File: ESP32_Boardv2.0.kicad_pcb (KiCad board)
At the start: 2 copper layers, 36 parts, among them IC1 AMS1117-3.3, IC2 CP2102N-A01-GQFN28, J1 USB_B_Micro, J2 Conn_01x19_Male, J3 Conn_01x19_Male, Q1 SS8050-G, Q2 SS8050-G, SW1 SW_Push, SW2 SW_Push, U1 ESP32-WROOM-32

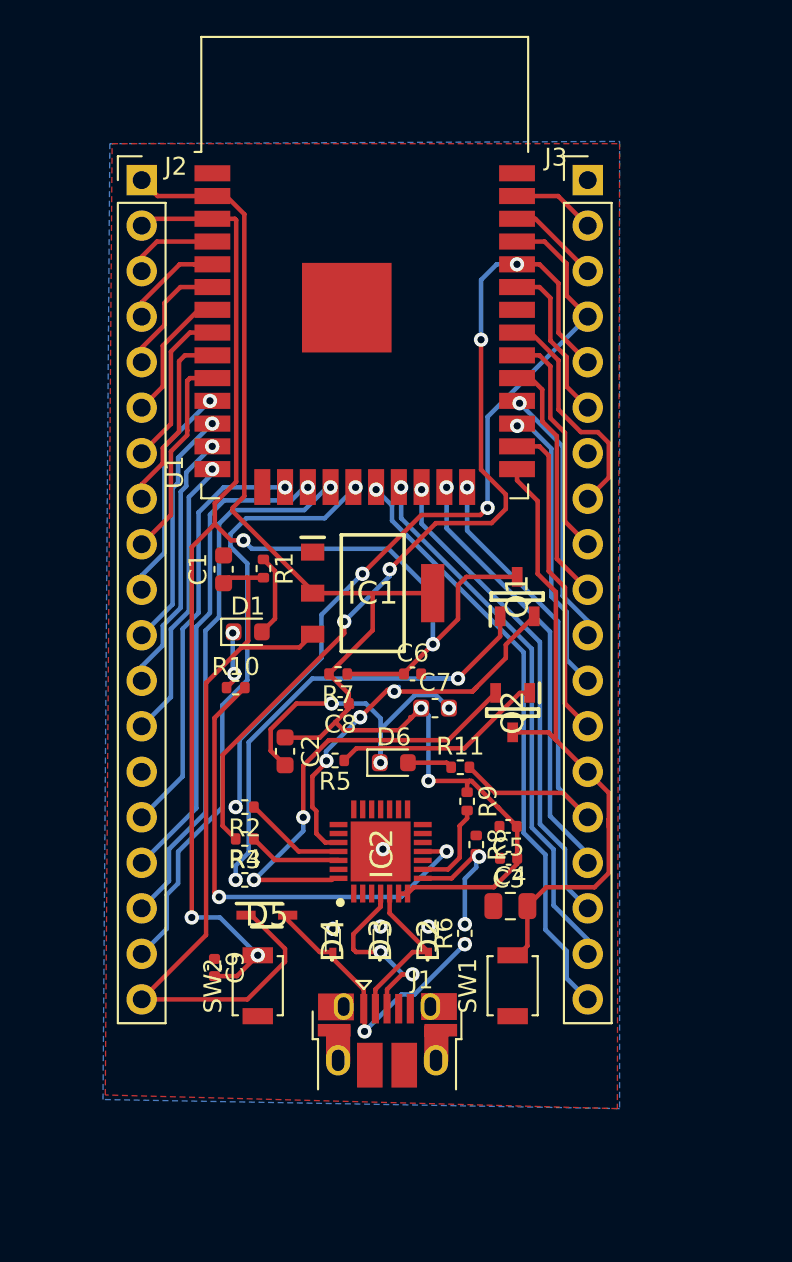
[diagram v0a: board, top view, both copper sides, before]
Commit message: 2 Layer PCB
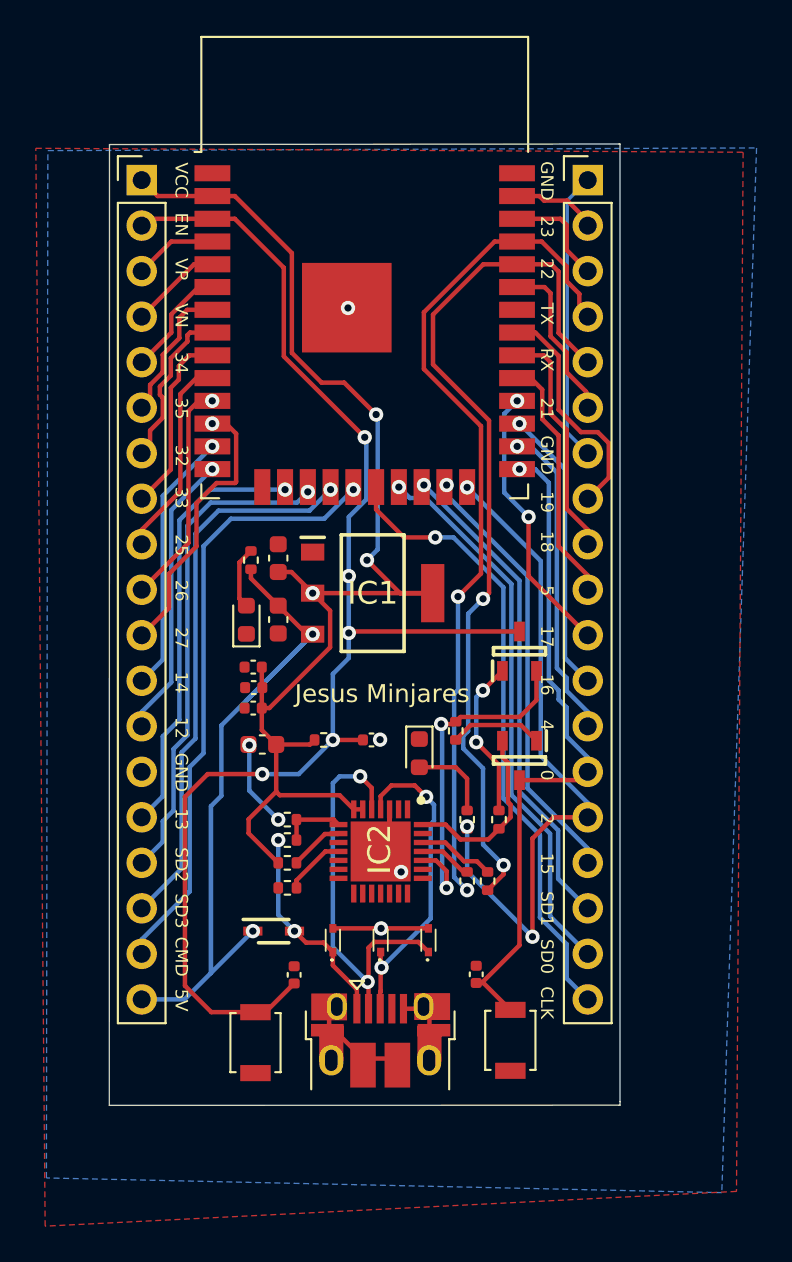
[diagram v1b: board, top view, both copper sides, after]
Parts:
- added G***: LOGO, UTEP_LOGO:UTEP LOGO 400x400, B.Cu at (117.7, 39.1)
- C4: footprint Capacitor_SMD:C_0805_2012Metric -> Capacitor_SMD:C_0402_1005Metric
- moved C3 17.1 mm to (110.5, 56.9)
- moved C5 16.8 mm to (110.5, 55.8)
- moved R4 14.6 mm to (124.2, 64.3), turned to 270 degrees
- moved R3 13.8 mm to (123.6, 67.7), turned to 270 degrees
- moved R2 13.1 mm to (122.4, 67.7), turned to 270 degrees
- moved C7 12.1 mm to (111.9, 49.7), turned to 90 degrees
- moved R10 11.5 mm to (112.4, 68.1)
- moved R6 11.2 mm to (112.4, 65.4), turned to 0 degrees
- moved R8 10.6 mm to (112.4, 64.3), turned to 0 degrees
- moved R9 10.6 mm to (112.4, 66.7), turned to 0 degrees
- moved R5 6.93 mm to (121.8, 59.3), turned to 90 degrees
- moved C8 4.86 mm to (110.5, 58.0)
- moved C9 4.46 mm to (112.8, 72.9)
- moved C6 4.34 mm to (117.1, 59.8)
- moved C4 4.26 mm to (122.9, 72.9), turned to 270 degrees
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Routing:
- net Net-(IC2-Pad11): track 27.6 -> 3.43 mm, vias 2 -> 0
- net GND: track 22.0 -> 42.2 mm, vias 9 -> 6
- net Net-(Q1-Pad1): track 27.6 -> 8.92 mm
- net /DTR: track 24.7 -> 10.2 mm, vias 2 -> 0
- net /USB_DN: track 9.06 -> 23.2 mm, vias 0 -> 2
- net /IO2: track 29.0 -> 37.9 mm, vias 1 -> 3
- net /USB_DP: track 10.5 -> 17.9 mm
- net Net-(Q2-Pad1): track 11.9 -> 5.21 mm
- net +5V: track 45.6 -> 39.5 mm, vias 0 -> 2
- net /EN: track 82.6 -> 77.0 mm, vias 4 -> 5
- net /VBUS: track 16.6 -> 11.8 mm
- net Net-(IC2-Pad8): track 7.66 -> 3.61 mm, vias 2 -> 0
- net /TXD0: track 44.2 -> 48.0 mm, vias 3 -> 2
- net /RTS: track 22.4 -> 19.3 mm, vias 3 -> 2
- net /RXD: track 5.75 -> 2.95 mm
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- added copper zone on F.Cu, net GND
- removed copper zone on F.Cu, net (none)
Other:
- board outline added: 28.5 x 53.6 mm
- board text added: "0"
- board text added: "12"
- board text added: "13"
- board text added: "14"
- board text added: "15"
- board text added: "16"
- board text added: "17"
- board text added: "18"
- board text added: "19"
- board text added: "2"
- board text added: "21"
- board text added: "22"
- board text added: "23"
- board text added: "25"
- board text added: "26"
- board text added: "27"
- board text added: "32"
- board text added: "33"
- board text added: "34"
- board text added: "35"
- board text added: "4"
- board text added: "5"
- board text added: "5V"
- board text added: "CLK"
- board text added: "CMD"
- board text added: "EN"
- board text added: "ESP32 Dev v1.0"
- board text added: "GND"
- board text added: "Jesus Minjares"
- board text added: "MS CPE"
- board text added: "RX"
- board text added: "SD0"
- board text added: "SD1"
- board text added: "SD2"
- board text added: "SD3"
- board text added: "TX"
- board text added: "VCC"
- board text added: "VN"
- board text added: "VP"
- board text added: "https://github.com/jminjares4"
